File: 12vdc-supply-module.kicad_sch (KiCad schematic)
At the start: 14 parts

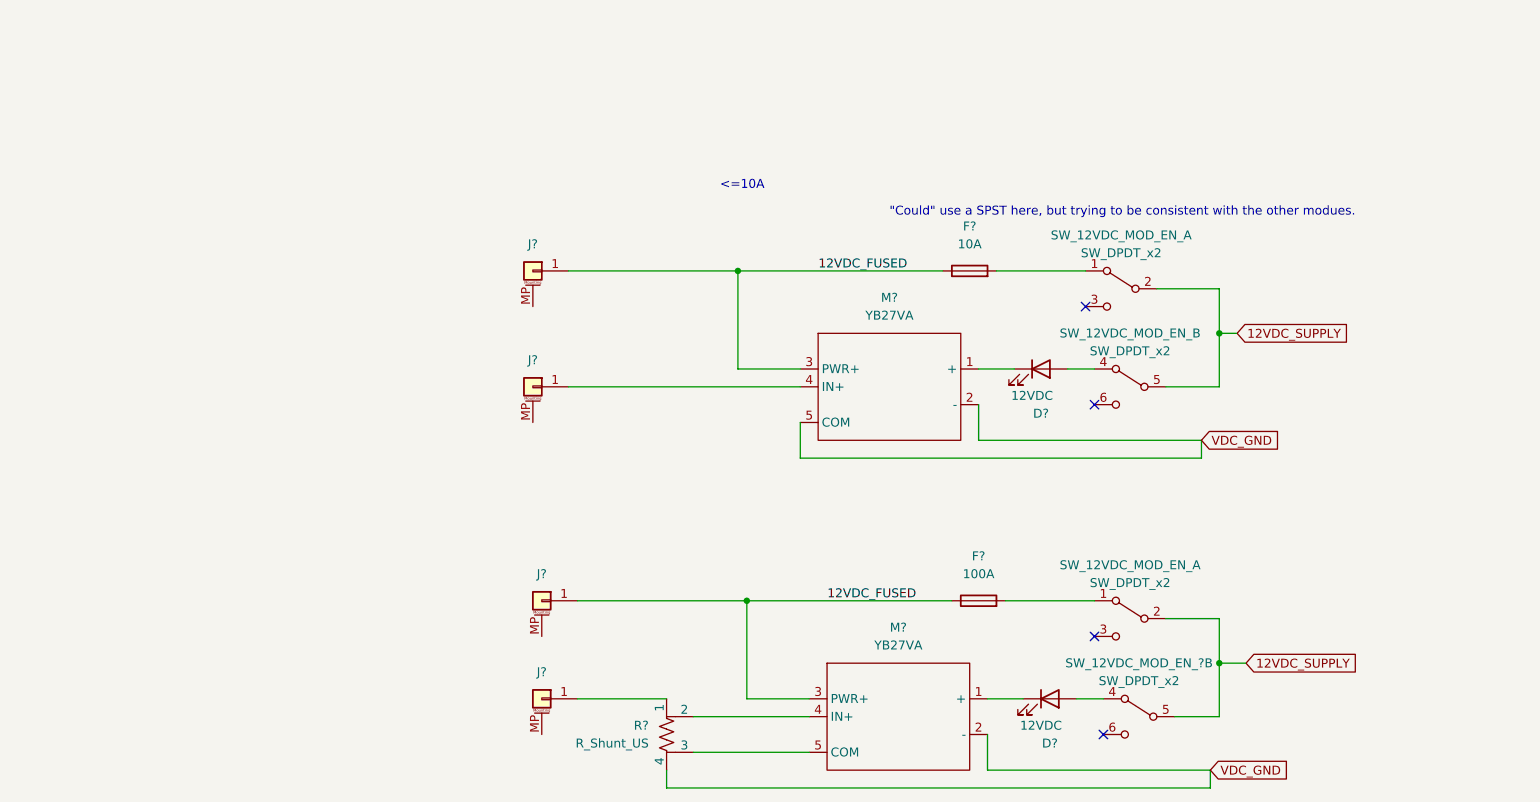
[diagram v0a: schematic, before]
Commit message: Bunch more changes
Blah blah
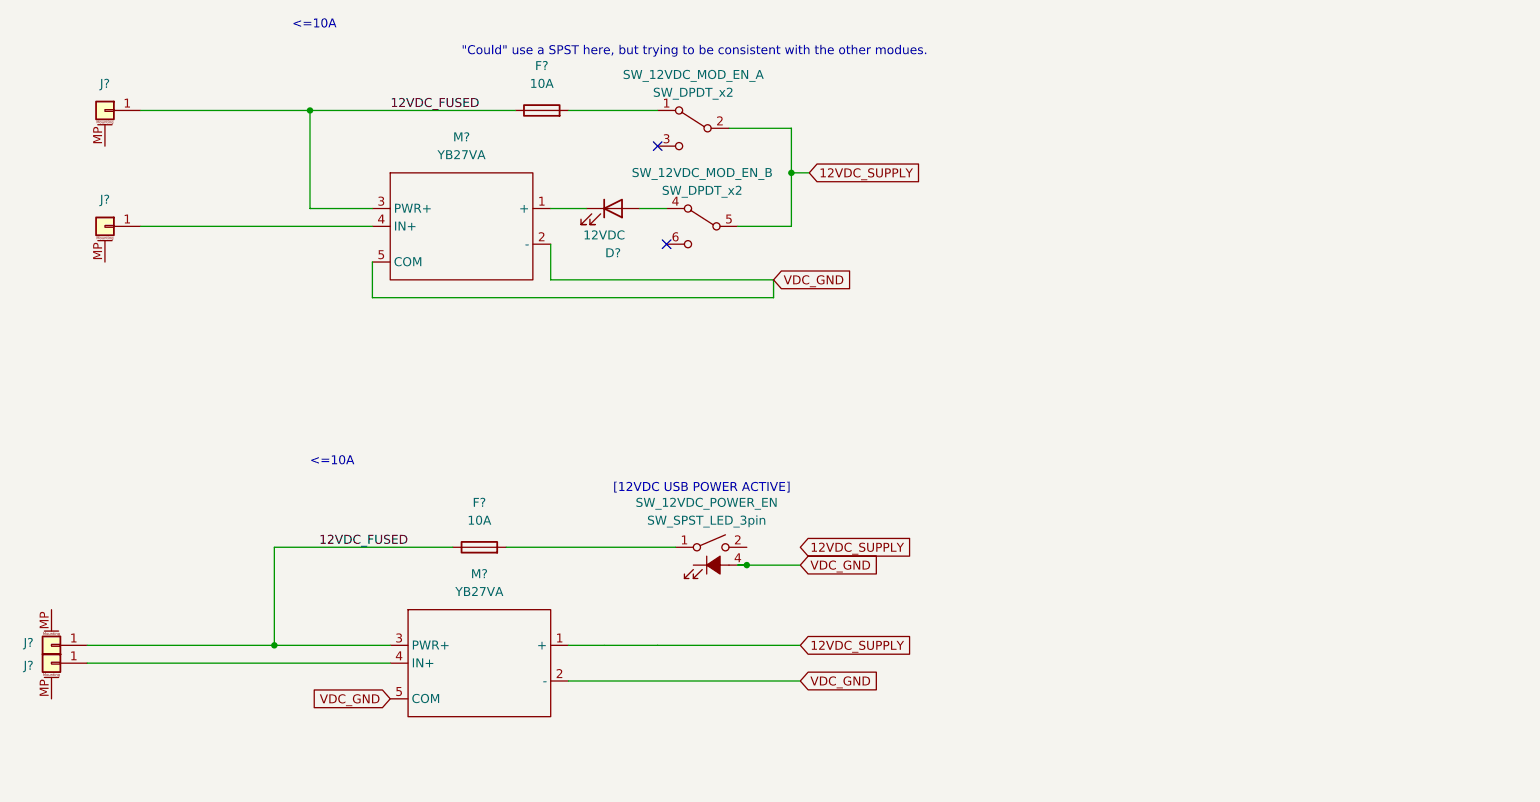
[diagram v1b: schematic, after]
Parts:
- removed D?: 12VDC, symbol Device:LED
- removed F?: 100A, symbol Device:Fuse
- removed J? (x2): Conn_01x01_MountingPin, symbol Connector_Generic_MountingPin:Conn_01x01_MountingPin
- removed M?: YB27VA, symbol bvm-library:5_Pin_Meter_With_Ext_Shunt
- removed R?: R_Shunt_US, symbol Device:R_Shunt_US
- removed SW_12VDC_MOD_EN_, SW_12VDC_MOD_EN_?: SW_DPDT_x2, symbol Switch:SW_DPDT_x2
- added F?: 10A, symbol Device:Fuse
- added J? (x2): Conn_01x01_MountingPin, symbol Connector_Generic_MountingPin:Conn_01x01_MountingPin
- added M?: YB27VA, symbol bvm-library:5_Pin_Meter_With_Ext_Shunt
- added SW_12VDC_POWER_EN: SW_SPST_LED_3pin, symbol bvm-library:SW_SPST_LED_3pin
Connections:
- net 12VDC_FUSED: now also F?.1, J?.1 (Pin_1), M?.3 (PWR+)
- net 12VDC_SUPPLY: now also M?.1 (+)
- net VDC_GND: now also M?.2 (-), M?.5 (COM), SW_12VDC_POWER_EN.4 (A)
- new net: J?.1 (Pin_1), M?.4 (IN+)
- new net: F?.2, SW_12VDC_POWER_EN.1
- no-connect marks 4 -> 2
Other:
- note added: "[12VDC USB POWER ACTIVE]"
- title: (none) -> Mr. Powers
- moved on the sheet: D?, F?, J?, M?, SW_12VDC_MOD_EN_A, SW_12VDC_MOD_EN_B
